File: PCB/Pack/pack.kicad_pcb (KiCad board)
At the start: 2 copper layers, 100 x 100 mm, 0 parts

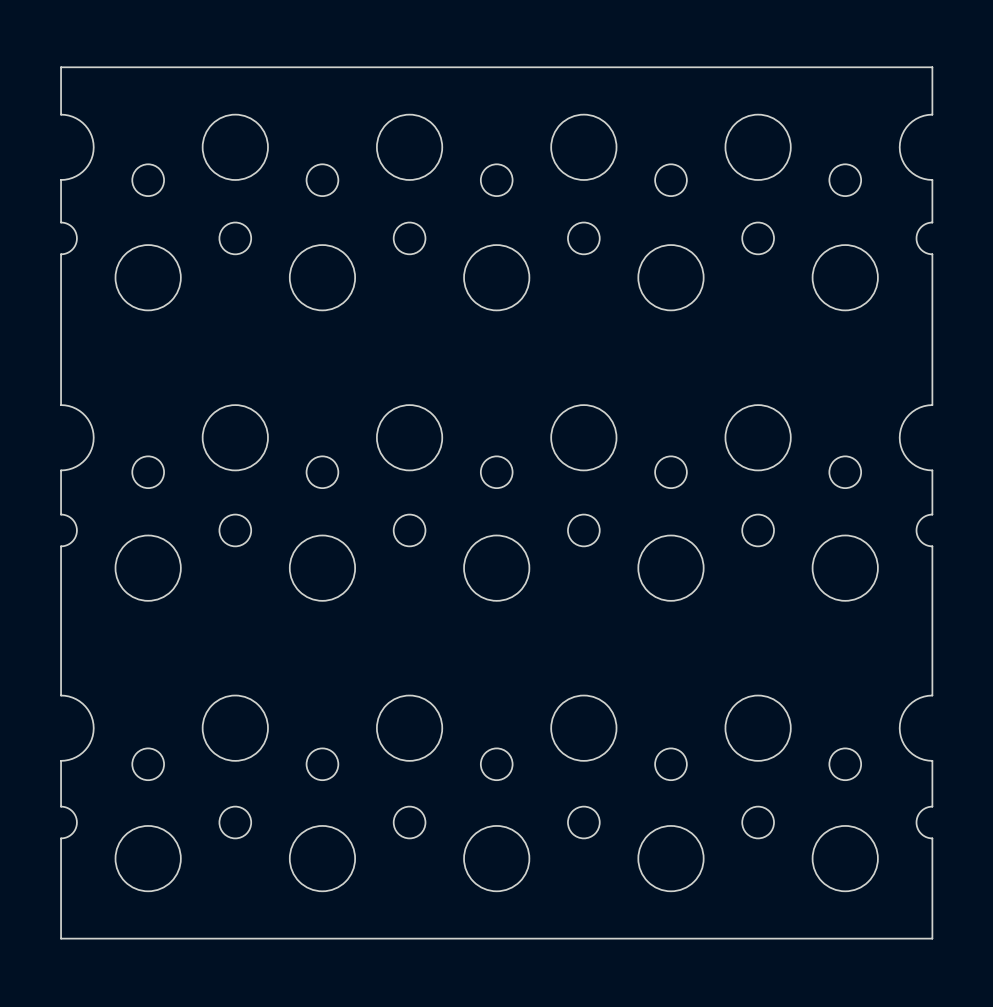
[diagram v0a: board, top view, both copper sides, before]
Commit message: pack schematic & pcb
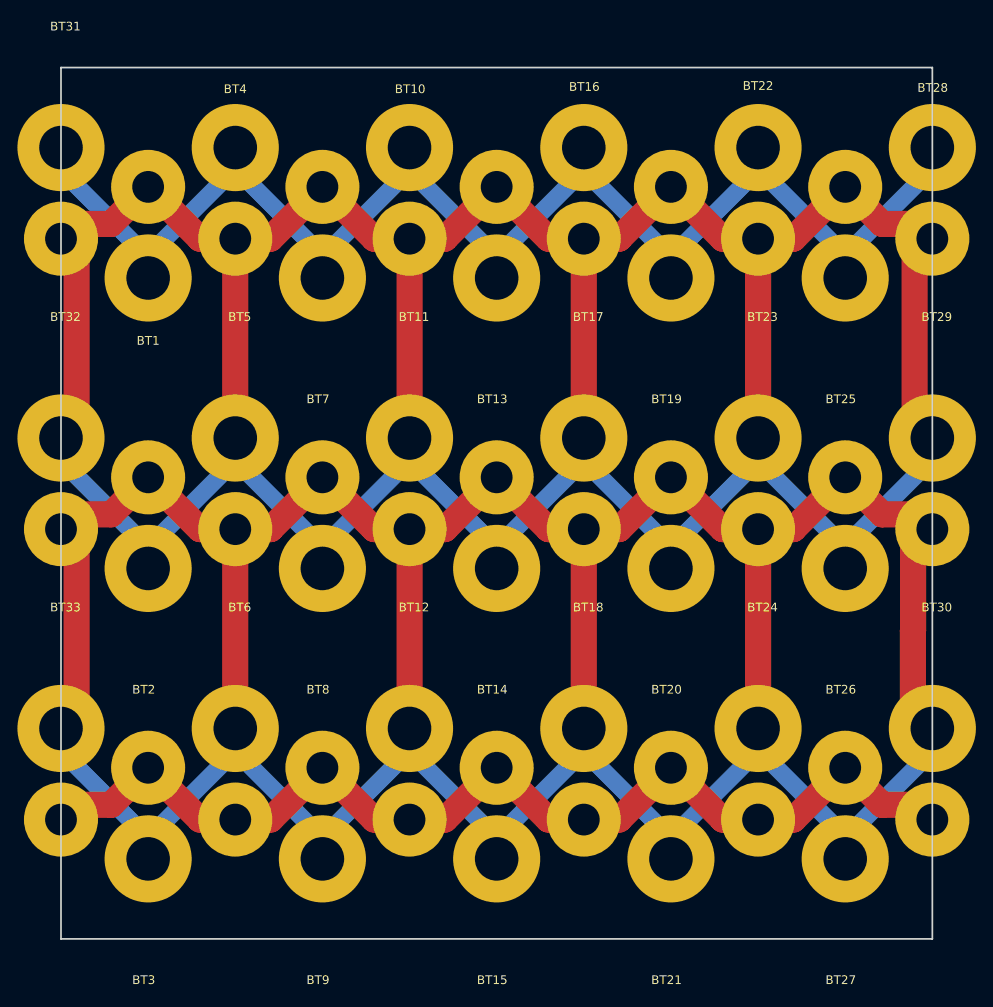
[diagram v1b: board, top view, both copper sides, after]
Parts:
- added BT1: Battery_Cell, ENNOID:Battery, F.Cu at (10.0, 24.2)
- added BT10: Battery_Cell, ENNOID:Battery, F.Cu at (40.0, 9.18)
- added BT11: Battery_Cell, ENNOID:Battery, F.Cu at (40.0, 42.5)
- added BT12: Battery_Cell, ENNOID:Battery, F.Cu at (40.0, 75.8)
- added BT13: Battery_Cell, ENNOID:Battery, F.Cu at (50.0, 24.2)
- added BT14: Battery_Cell, ENNOID:Battery, F.Cu at (50.0, 57.5)
- added BT15: Battery_Cell, ENNOID:Battery, F.Cu at (50.0, 90.8)
- added BT16: Battery_Cell, ENNOID:Battery, F.Cu at (60.0, 9.18)
- added BT17: Battery_Cell, ENNOID:Battery, F.Cu at (60.0, 42.5)
- added BT18: Battery_Cell, ENNOID:Battery, F.Cu at (60.0, 75.8)
- added BT19: Battery_Cell, ENNOID:Battery, F.Cu at (70.0, 24.2)
- added BT2: Battery_Cell, ENNOID:Battery, F.Cu at (10.0, 57.5)
- added BT20: Battery_Cell, ENNOID:Battery, F.Cu at (70.0, 57.5)
- added BT21: Battery_Cell, ENNOID:Battery, F.Cu at (70.0, 90.8)
- added BT22: Battery_Cell, ENNOID:Battery, F.Cu at (80.0, 9.18)
- added BT23: Battery_Cell, ENNOID:Battery, F.Cu at (80.0, 42.5)
- added BT24: Battery_Cell, ENNOID:Battery, F.Cu at (80.0, 75.8)
- added BT25: Battery_Cell, ENNOID:Battery, F.Cu at (90.0, 24.2)
- added BT26: Battery_Cell, ENNOID:Battery, F.Cu at (90.0, 57.5)
- added BT27: Battery_Cell, ENNOID:Battery, F.Cu at (90.0, 90.8)
- added BT28: Battery_Cell, ENNOID:Battery, F.Cu at (100.0, 9.18)
- added BT29: Battery_Cell, ENNOID:Battery, F.Cu at (100.0, 42.5)
- added BT3: Battery_Cell, ENNOID:Battery, F.Cu at (10.0, 90.8)
- added BT30: Battery_Cell, ENNOID:Battery, F.Cu at (100.0, 75.8)
- added BT31: Battery_Cell, ENNOID:Battery, F.Cu at (0.00, 9.18)
- added BT32: Battery_Cell, ENNOID:Battery, F.Cu at (0.00, 42.5)
- added BT33: Battery_Cell, ENNOID:Battery, F.Cu at (0.00, 75.8)
- added BT4: Battery_Cell, ENNOID:Battery, F.Cu at (20.0, 9.18)
- added BT5: Battery_Cell, ENNOID:Battery, F.Cu at (20.0, 42.5)
- added BT6: Battery_Cell, ENNOID:Battery, F.Cu at (20.0, 75.8)
- added BT7: Battery_Cell, ENNOID:Battery, F.Cu at (30.0, 24.2)
- added BT8: Battery_Cell, ENNOID:Battery, F.Cu at (30.0, 57.5)
- added BT9: Battery_Cell, ENNOID:Battery, F.Cu at (30.0, 90.8)
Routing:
- net Net-(BT11-Pad2): track 0.00 -> 415.0 mm
- net Net-(BT1-Pad2): track 0.00 -> 412.5 mm
- net Net-(BT1-Pad1): track 0.00 -> 167.5 mm
- net Net-(BT12-Pad2): track 0.00 -> 119.6 mm
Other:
- outline, holes or cut-outs redrawn
- rule pad_to_mask_clearance: 0.2 -> 0.051
